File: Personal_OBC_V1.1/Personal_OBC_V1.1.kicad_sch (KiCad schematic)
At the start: 30 parts, among them IC1 AP2205-33W5-7, J2 PYRO CHANNELS, J3 POWER IN, J4 PROG PINS, J4 USB_B_Micro, SW1 SW_SPDT, U1 STM32F302K8Ux, U2 MS560702BA03-50, U3 W25X40CLUXIG_TR, X1 ECS-2520MV-xxx-xx

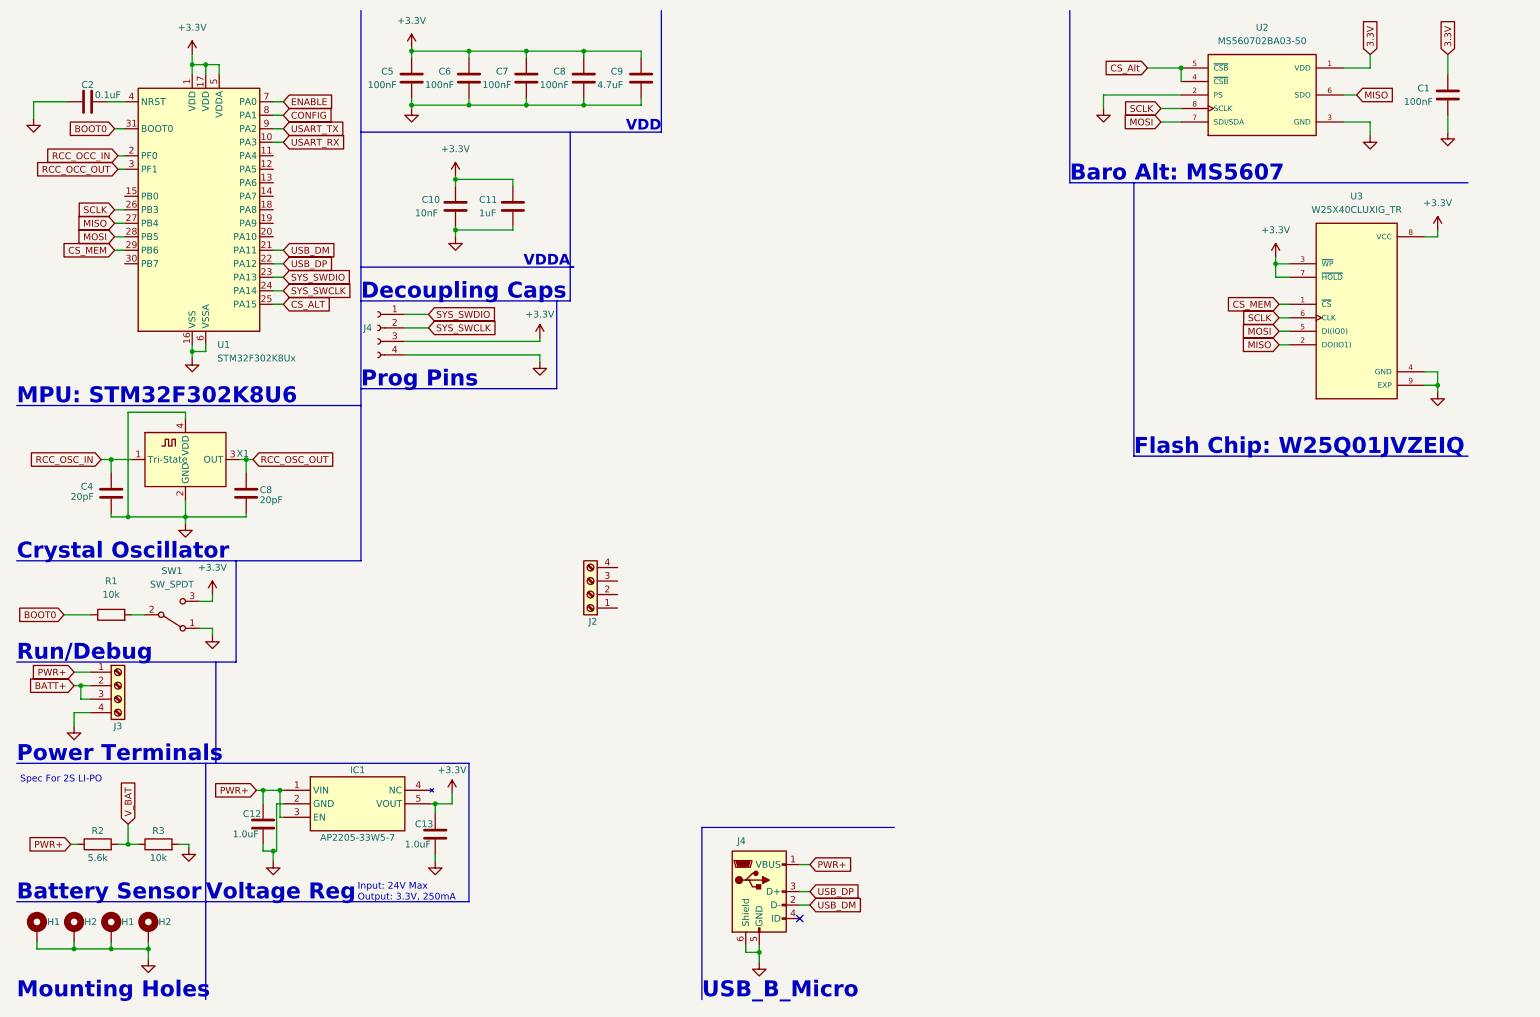
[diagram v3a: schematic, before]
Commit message: Reworked schematic
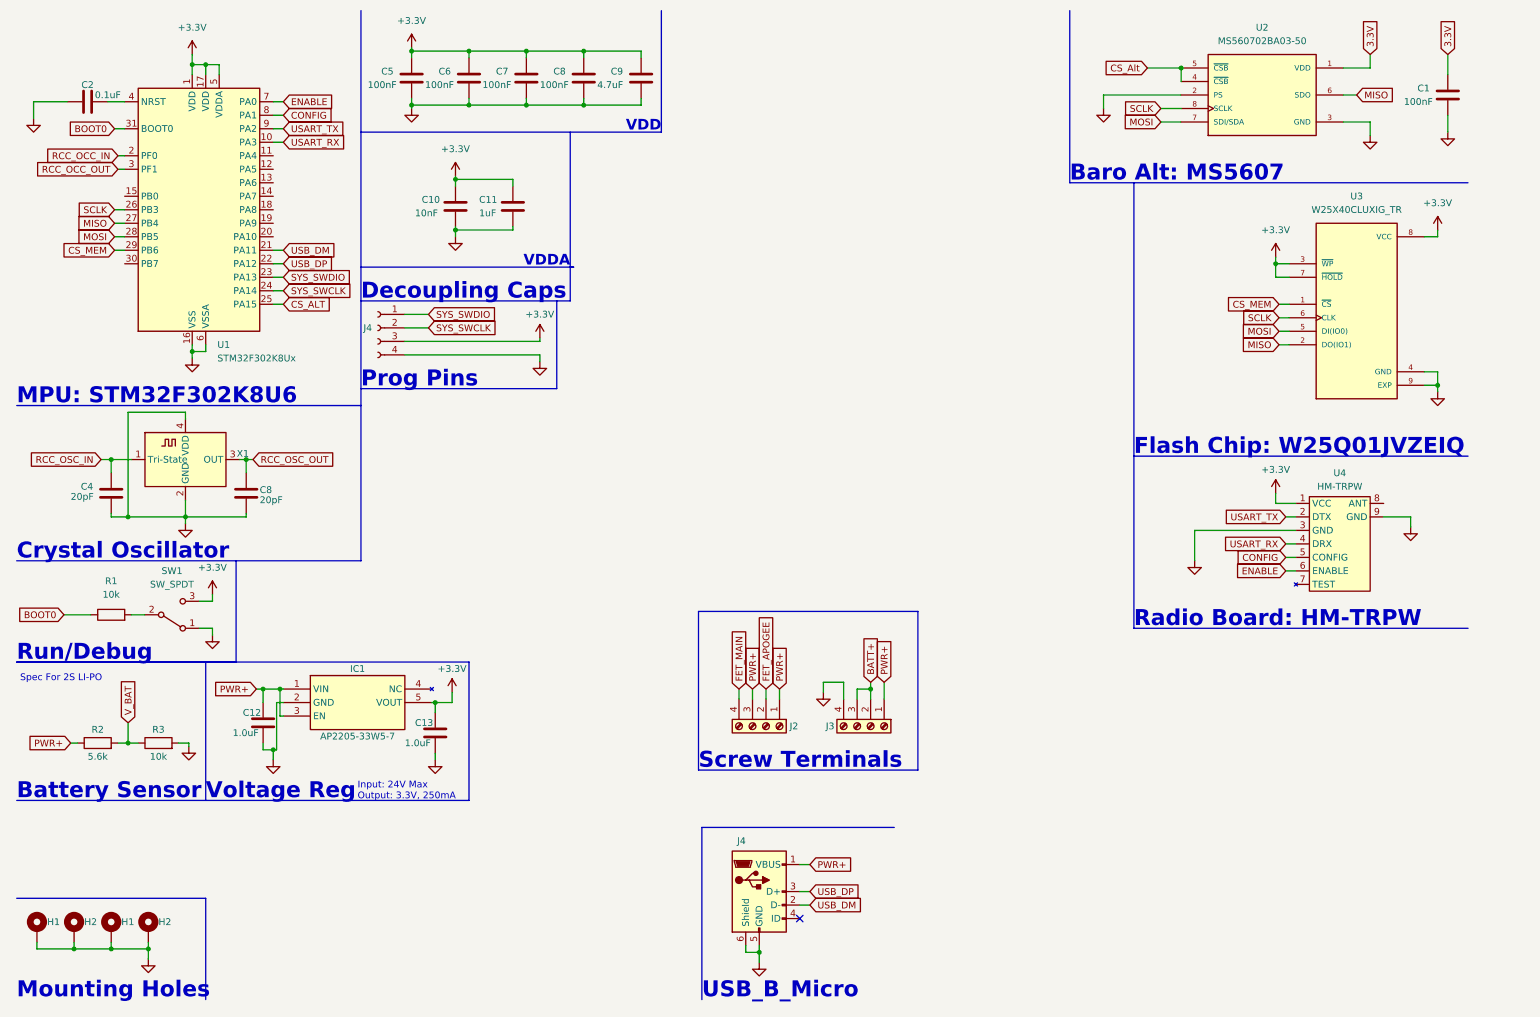
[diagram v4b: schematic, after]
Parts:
- added U4: HM-TRPW, HW-TRPW:HM-TRPW, symbol HW-TRPW:HW-TRPW
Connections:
- net +3.3V: now also U4.1 (VCC)
- net CONFIG: now also U4.5 (CONFIG)
- net ENABLE: now also U4.6 (ENABLE)
- net GND: now also U4.3 (GND), U4.9 (GND)
- net PWR+: now also J2.1 (Pin_1), J2.3 (Pin_3)
- net USART_RX: now also U4.4 (DRX)
- net USART_TX: now also U4.2 (DTX)
- net FET_APOGEE: now reaches J2.2 (Pin_2)
- net FET_MAIN: now reaches J2.4 (Pin_4)
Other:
- note added: "Radio Board: HM-TRPW"
- note added: "Screw Terminals"
- note removed: "Power Terminals"
- moved on the sheet: C12, C13, IC1, J2, J3, R2, R3

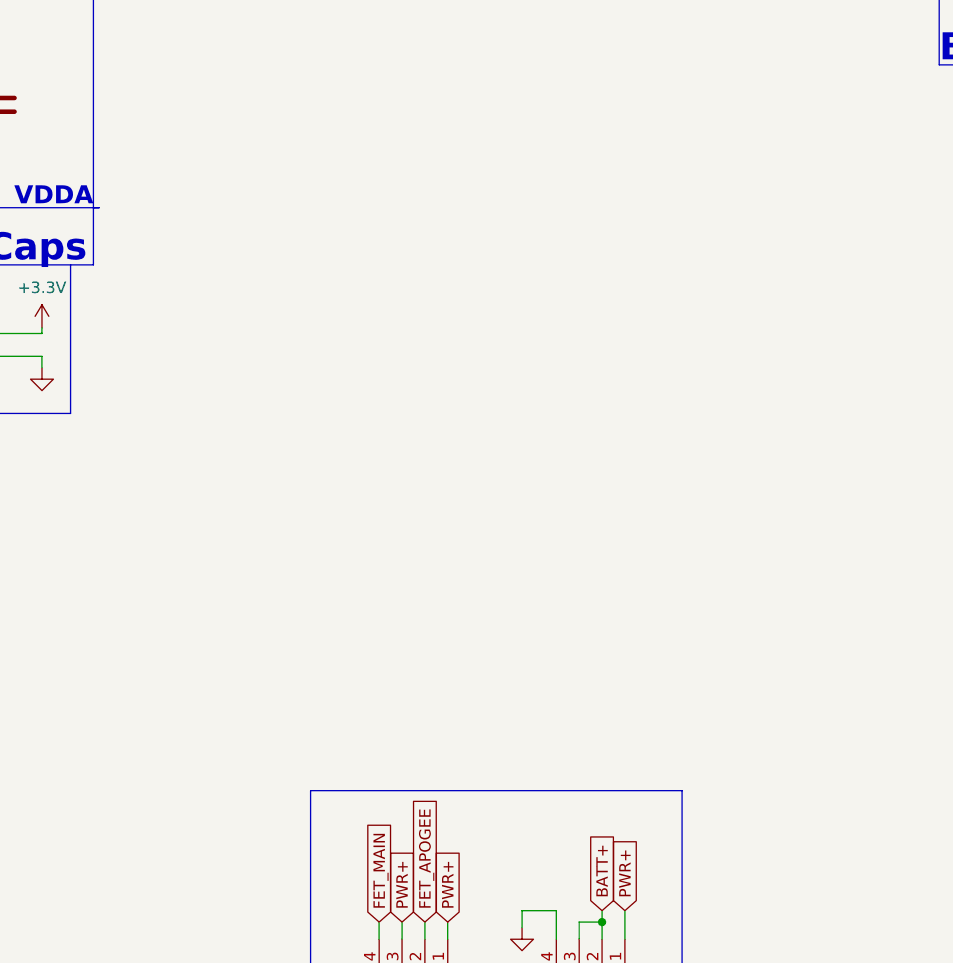
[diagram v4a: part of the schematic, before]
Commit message: Sent
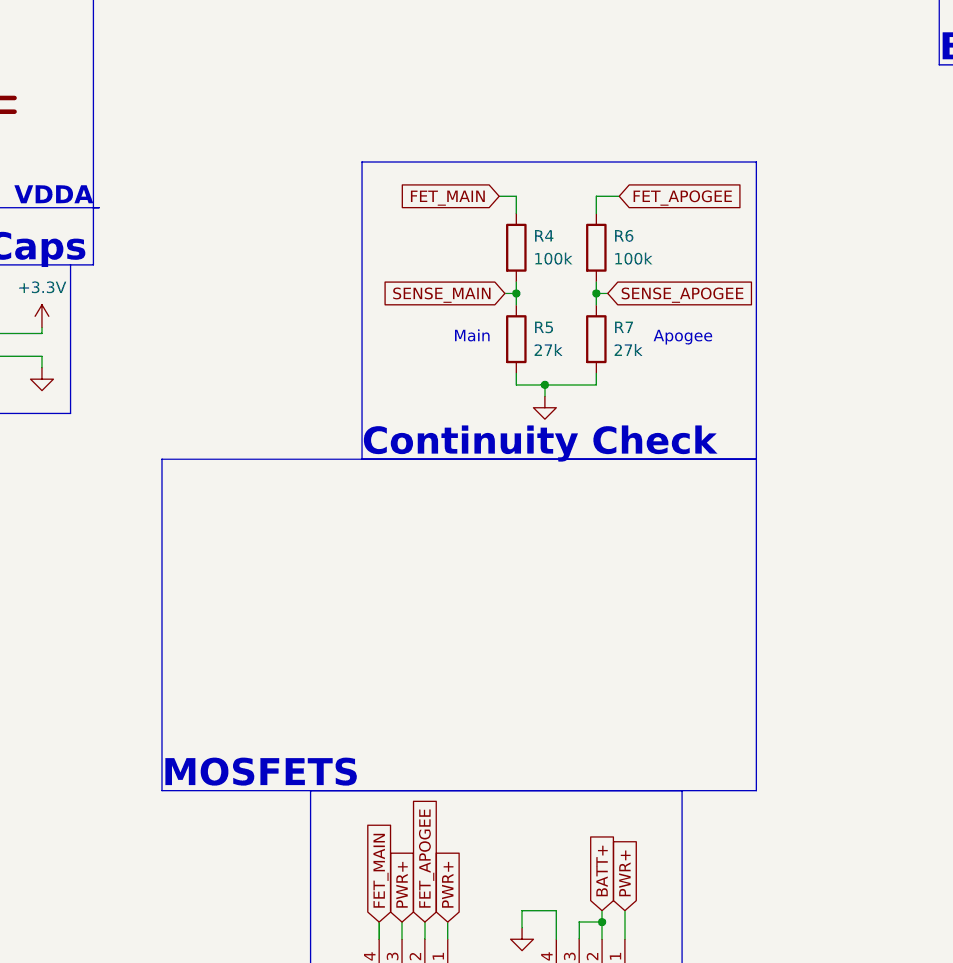
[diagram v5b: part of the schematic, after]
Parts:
- added R4, R6: 100k, symbol Device:R
- added R5, R7: 27k, symbol Device:R
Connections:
- net FET_APOGEE: now also R6.1
- net FET_MAIN: now also R4.1
- net GND: now also R5.2, R7.2
- new net SENSE_APOGEE: R6.2, R7.1
- new net SENSE_MAIN: R4.2, R5.1
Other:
- note added: "Apogee"
- note added: "Continuity Check"
- note added: "MOSFETS"
- note added: "Main"

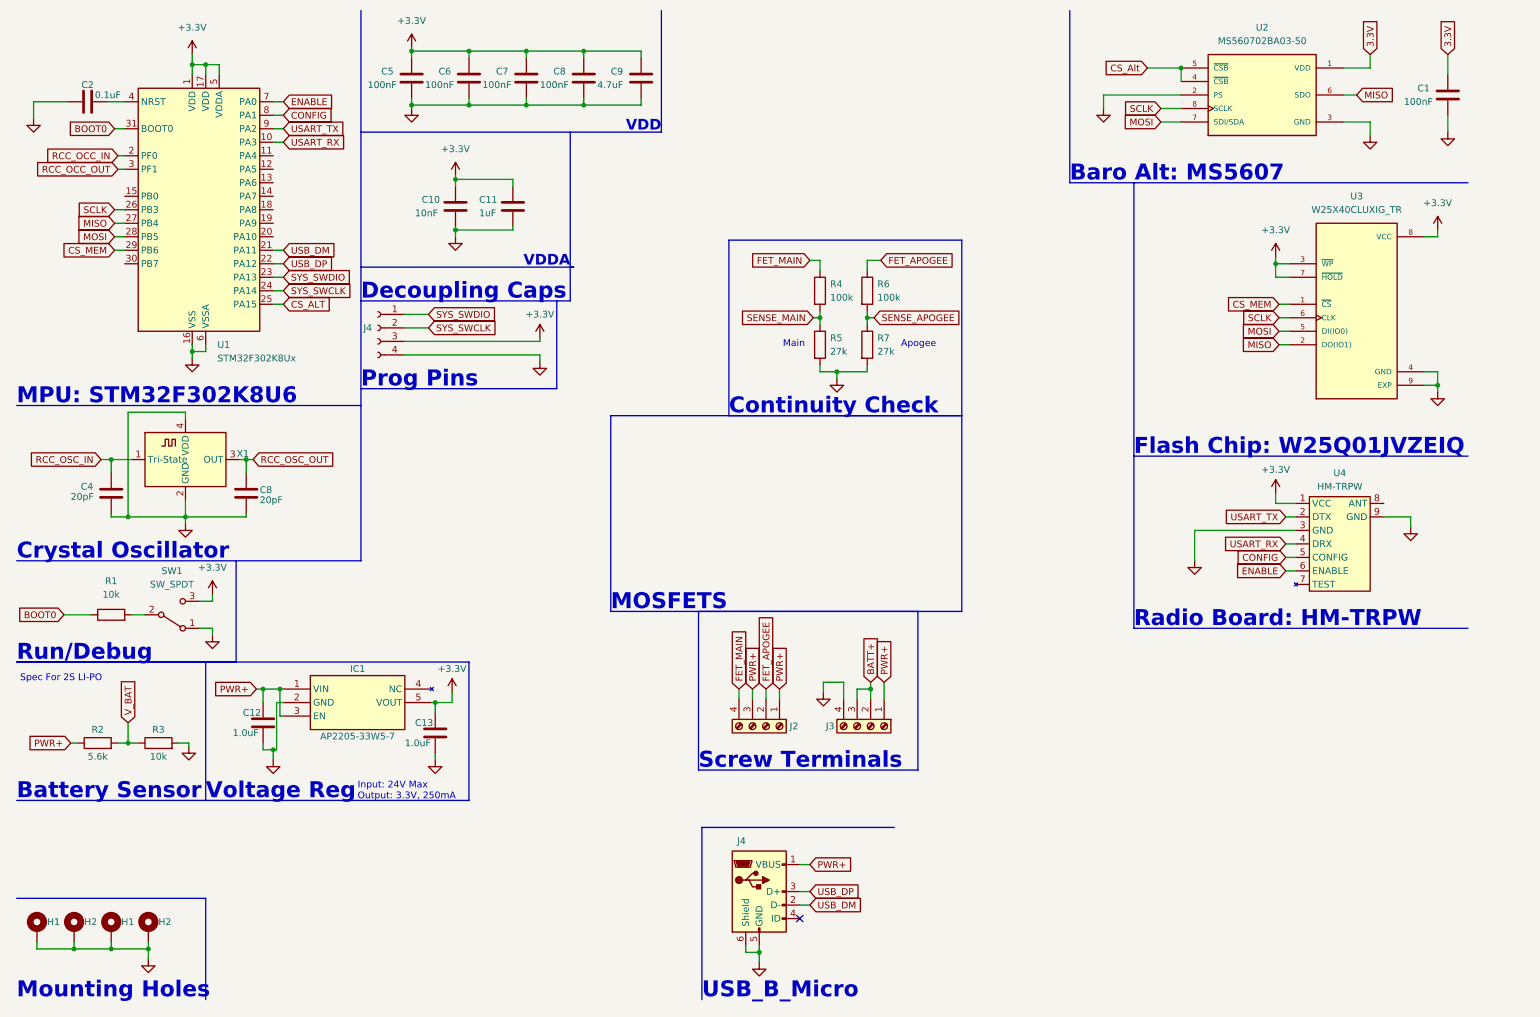
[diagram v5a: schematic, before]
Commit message: Mosfets Required
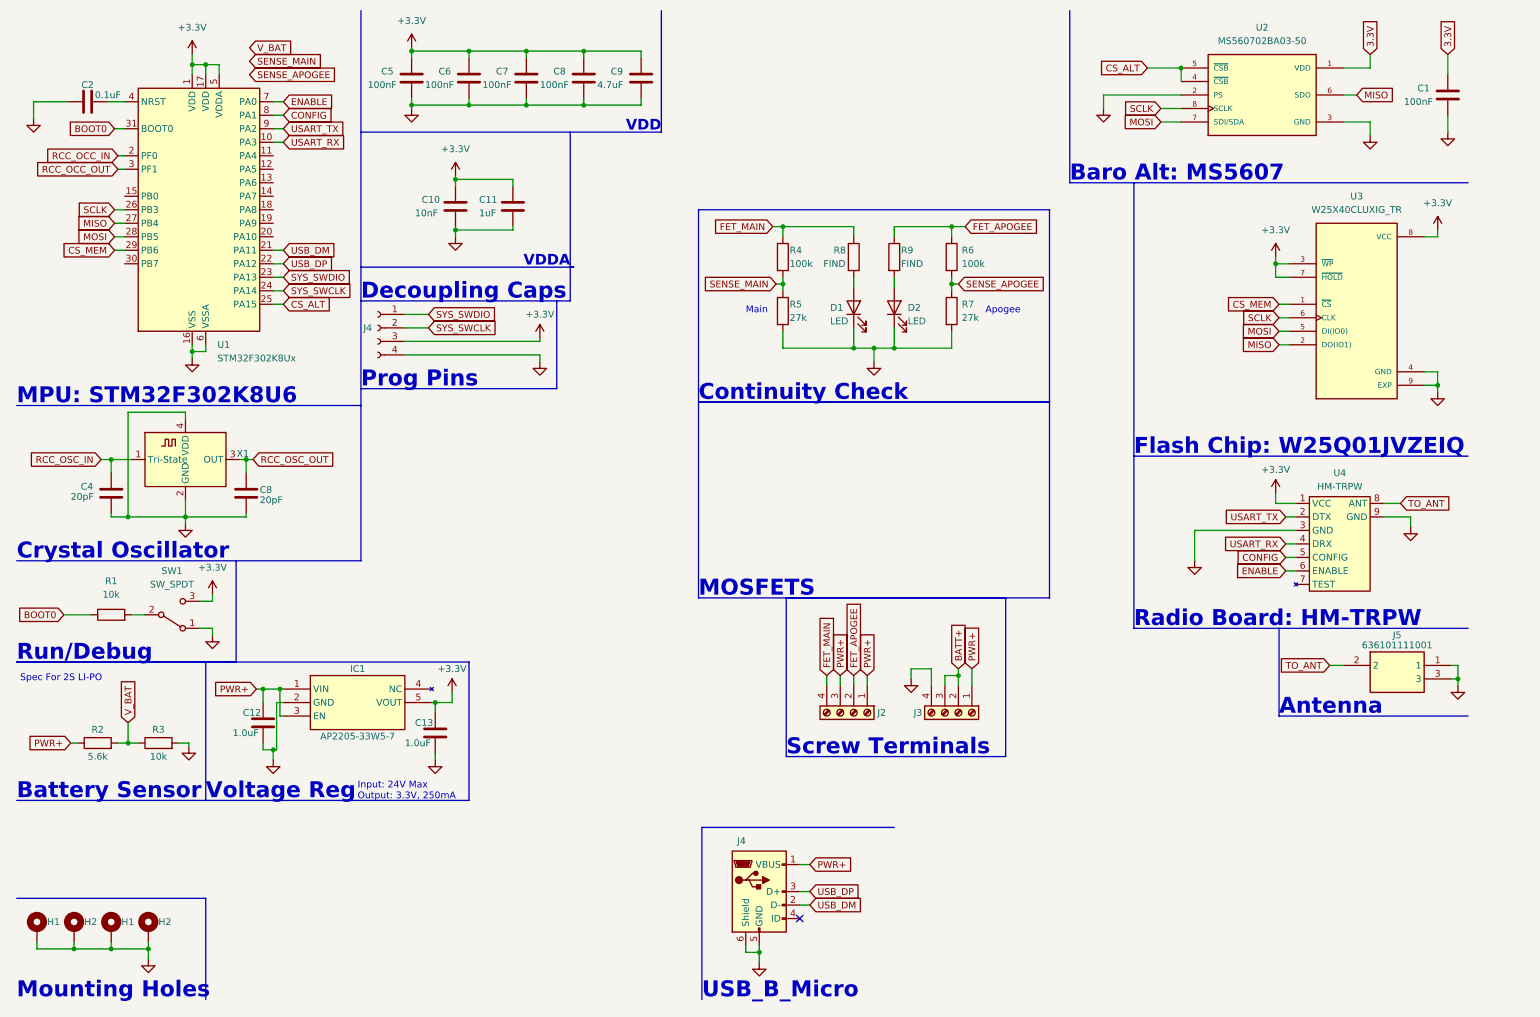
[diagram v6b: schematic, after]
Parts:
- added D1, D2: LED, symbol Device:LED
- added J5: 636101111001, 636101111001, symbol 636101111001:636101111001
- added R8, R9: FIND, symbol Device:R
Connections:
- net CS_Alt is gone; now on net CS_ALT: U2.4 (~{CSB}), U2.5 (~{CSB})
- net FET_APOGEE: now also R9.1
- net FET_MAIN: now also R8.1
- net GND: now also D1.1 (K), D2.1 (K), J5.1, J5.3
- net TO_ANT: now reaches U4.8 (ANT)
- net TO_ANT: now also J5.2
- new net: D1.2 (A), R8.2
- new net: D2.2 (A), R9.2
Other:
- note added: "Antenna"
- moved on the sheet: J2, J3, R4, R5, R6, R7
